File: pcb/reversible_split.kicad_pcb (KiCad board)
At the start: 2 copper layers, 134 x 93.8 mm, 22 parts

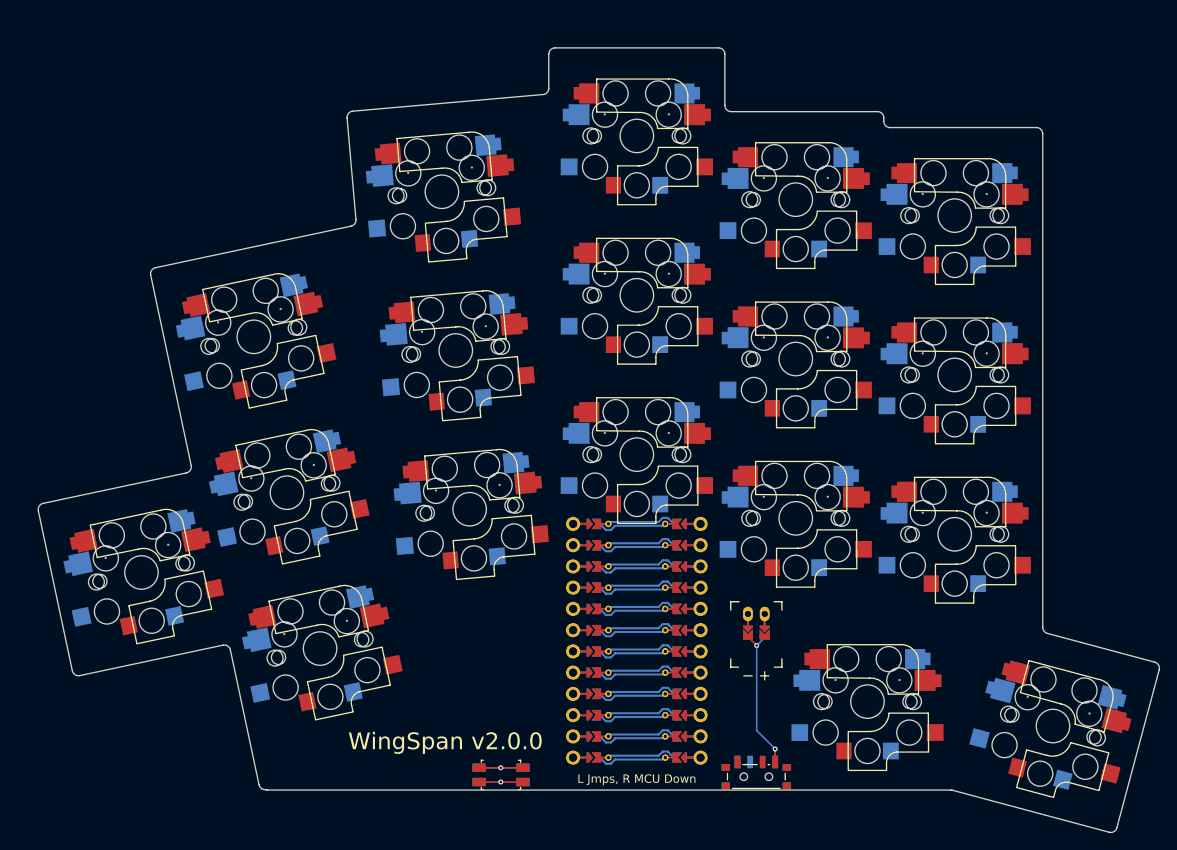
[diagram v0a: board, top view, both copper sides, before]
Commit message: Routed quick and dirty
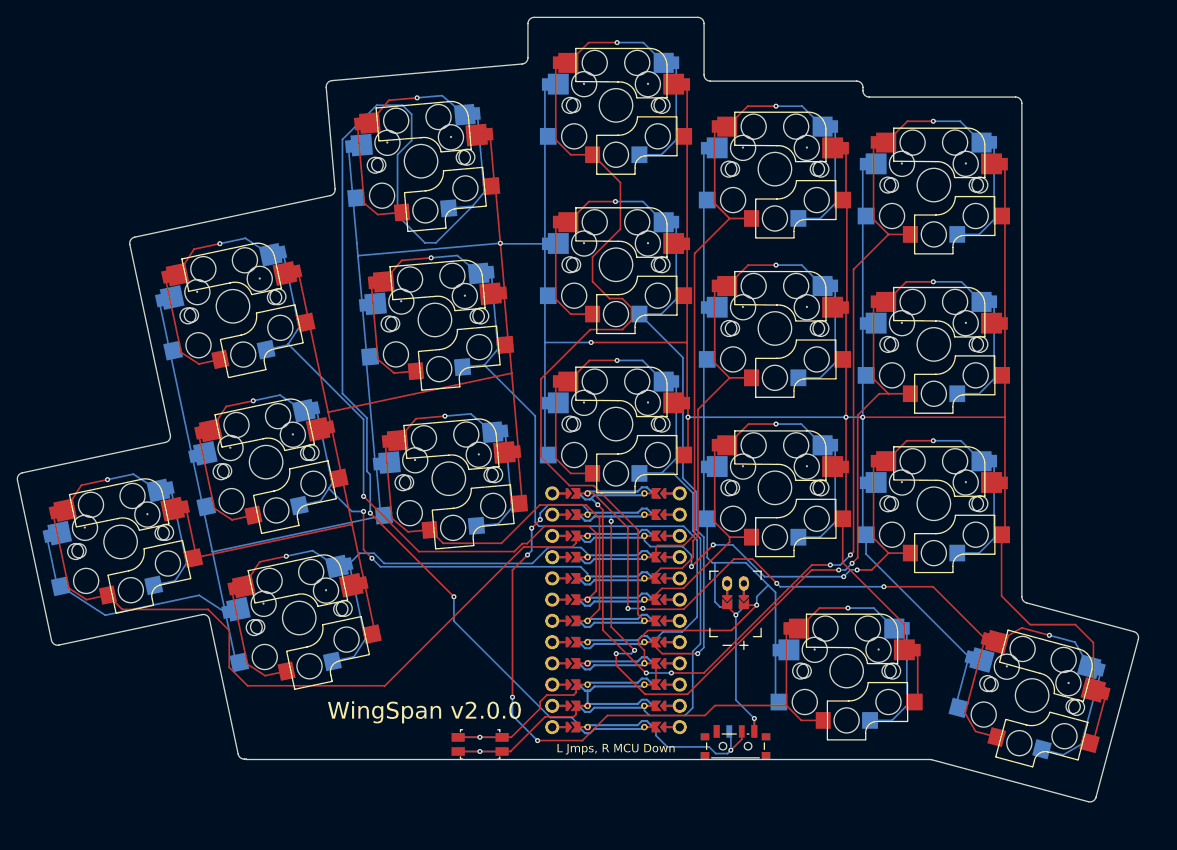
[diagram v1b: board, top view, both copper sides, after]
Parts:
- moved RST1 4.42 mm to (165.5, 127.8)
- moved S7 4.42 mm to (158.5, 58.1)
- moved S1 4.42 mm to (122.5, 103.6)
- moved S17 4.42 mm to (209.3, 119.1)
- moved S5 4.42 mm to (161.8, 96.1)
- moved S12 4.42 mm to (200.8, 78.1)
- moved S3 4.42 mm to (139.9, 94.1)
- moved MCU1 4.42 mm to (181.8, 113.1)
- moved S11 4.42 mm to (200.8, 97.2)
- moved S13 4.42 mm to (200.8, 59.1)
- moved S18 4.42 mm to (231.5, 122.0)
- moved PWR1 4.42 mm to (196.1, 128.0)
- moved S2 4.42 mm to (143.9, 112.7)
- moved S15 4.42 mm to (219.8, 80.0)
- moved S8 4.42 mm to (181.8, 89.6)
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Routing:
- net GND: track 40.0 -> 839.1 mm, vias 1 -> 7
- net matrix_ring_top: track 9.84 -> 171.0 mm, vias 0 -> 3
- net matrix_inner_top: track 9.84 -> 146.3 mm, vias 0 -> 6
- net matrix_inner_home: track 9.84 -> 131.7 mm, vias 0 -> 6
- net matrix_middle_top: track 9.84 -> 126.8 mm, vias 0 -> 1
- net matrix_outer_home: track 9.83 -> 123.0 mm, vias 0 -> 1
- net thumb_tucky: track 9.83 -> 120.2 mm, vias 0 -> 6
- net thumb_reachy: track 9.83 -> 117.3 mm, vias 0 -> 5
- net matrix_pinky_top: track 9.83 -> 114.5 mm, vias 0 -> 2
- net matrix_ring_home: track 9.83 -> 109.1 mm, vias 0 -> 1
- net matrix_middle_home: track 9.84 -> 102.0 mm, vias 0 -> 2
- net matrix_index_top: track 9.84 -> 98.0 mm, vias 0 -> 1
- net matrix_middle_bottom: track 9.84 -> 92.8 mm, vias 0 -> 1
- net matrix_pinky_home: track 9.83 -> 90.3 mm, vias 0 -> 3
- net matrix_ring_bottom: track 9.83 -> 88.3 mm, vias 0 -> 1
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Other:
- outline, holes or cut-outs redrawn
